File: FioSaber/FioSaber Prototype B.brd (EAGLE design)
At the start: 26.7 x 44.7 mm, 18 parts, among them P1 WIICHUCK, T1 2N2222

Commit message: labeled motor header
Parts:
- renumbered U$2 to MOTOR
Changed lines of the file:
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@@
 <element name="R4" library="adafruit" package="0207/7" value="33Ω" x="13.97" y="27.94" rot="R270"/>
 <element name="R3" library="adafruit" package="0207/7" value="1kΩ" x="11.43" y="27.94" rot="R90"/>
-<element name="U$2" library="headers(.1in)" package="1X2" value="1X2" x="11.43" y="35.56"/>
+<element name="MOTOR" library="headers(.1in)" package="1X2" value="1X2" x="11.43" y="35.56"/>
 <element name="D1" library="adafruit" package="DO41-10" value="1N4004" x="6.35" y="17.145" rot="R90"/>
 <element name="S1" library="adafruit" package="EG1218" value="" x="12.7" y="17.145" rot="R90"/>
@@
 <signal name="N$19">
 <contactref element="T1" pad="C"/>
-<contactref element="U$2" pad="1"/>
+<contactref element="MOTOR" pad="1"/>
 <contactref element="D2" pad="A"/>
 <contactref element="C1" pad="2"/>
@@
 </signal>
 <signal name="N$20">
-<contactref element="U$2" pad="2"/>
+<contactref element="MOTOR" pad="2"/>
 <contactref element="R4" pad="2"/>
 <contactref element="D2" pad="C"/>

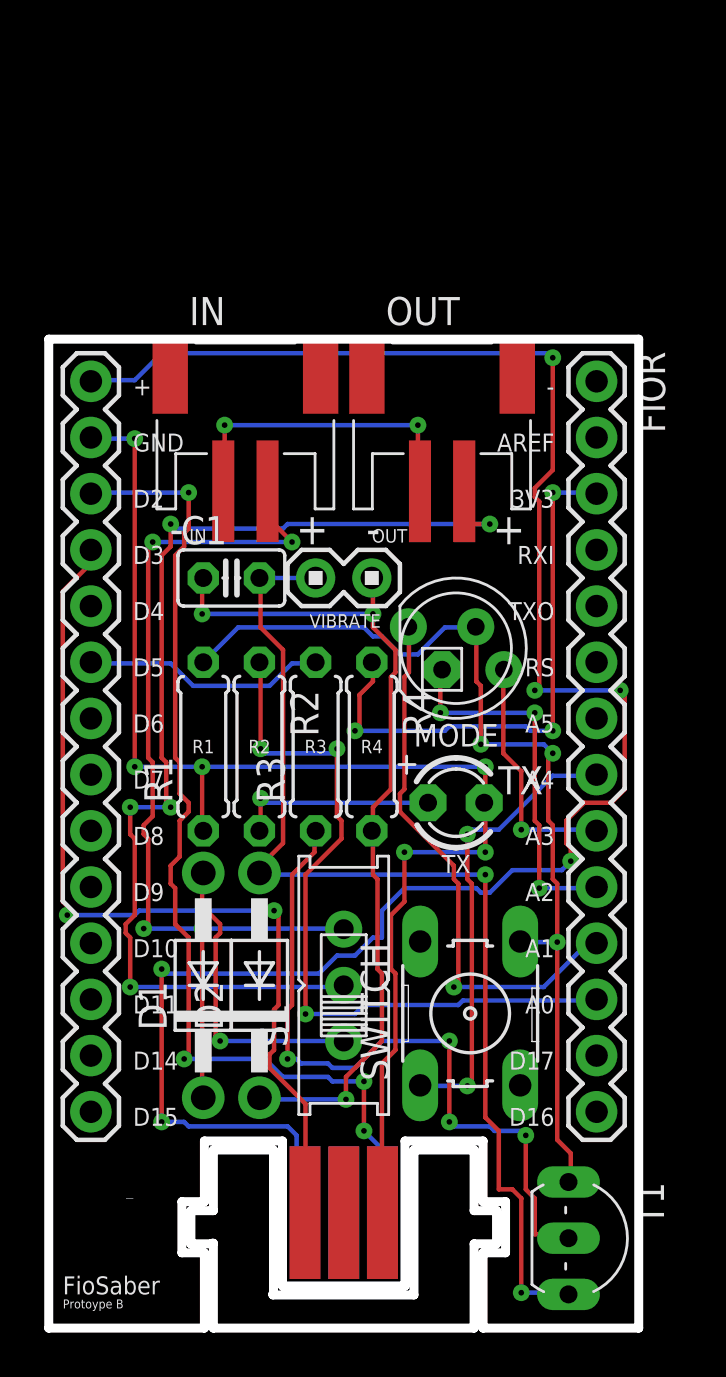
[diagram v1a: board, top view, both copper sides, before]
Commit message: reconfigured prototype b
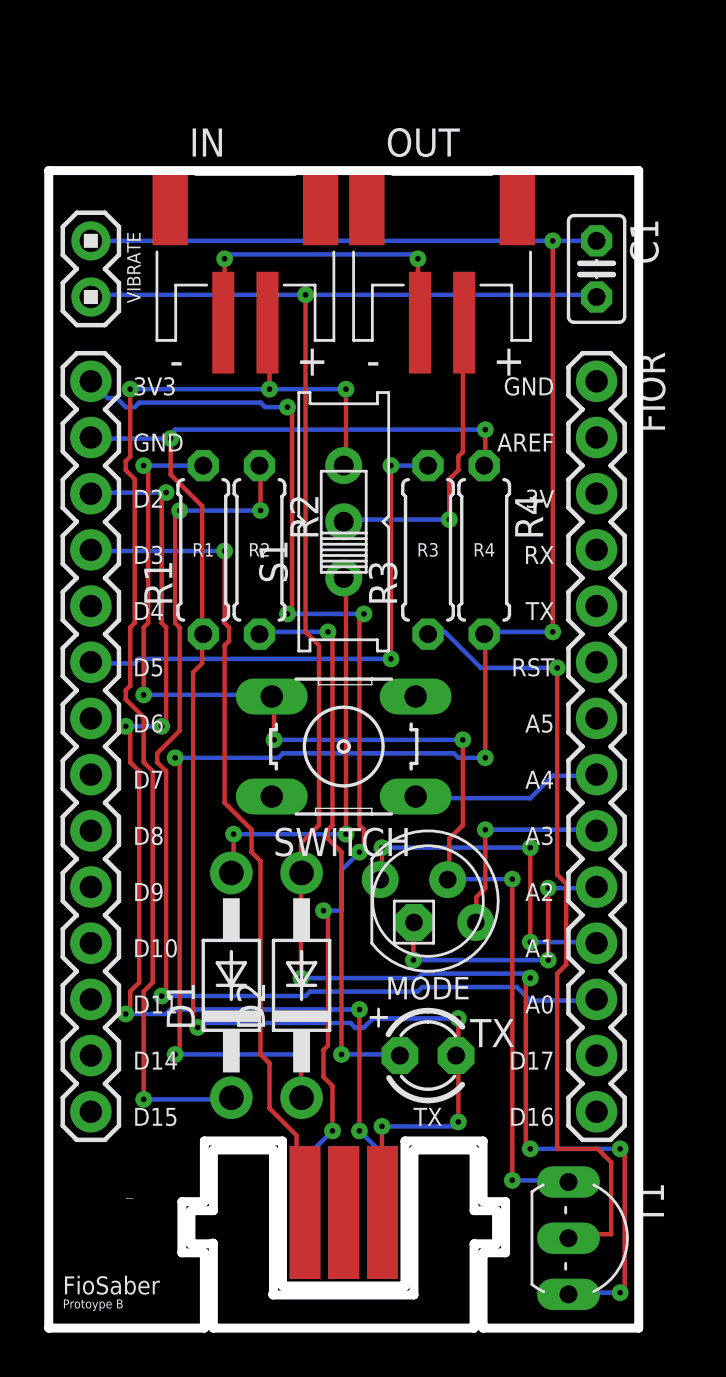
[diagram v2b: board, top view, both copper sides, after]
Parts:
- moved C1 21.6 mm to (24.1, 49.5), turned to 270 degrees
- moved S1 21.0 mm to (12.7, 38.1)
- moved MOTOR 16.3 mm to (1.27, 48.3), turned to 90 degrees
- moved SWITCH 13.4 mm to (12.7, 27.9), turned to 180 degrees
- moved MODE 11.5 mm to (16.5, 21.0)
- moved TX 11.5 mm to (16.5, 14.0)
- moved R3 10.2 mm to (16.5, 36.8)
- moved R4 10.2 mm to (19.1, 36.8)
- moved R1 8.89 mm to (6.35, 36.8)
- moved R2 8.89 mm to (8.89, 36.8)
- moved IN 7.62 mm to (8.26, 50.8)
- moved OUT 7.62 mm to (17.1, 50.8)
- moved D2 1.90 mm to (10.8, 17.1)
- moved D1 1.27 mm to (7.62, 17.1)
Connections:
- removed net N$12: FIOR.3, R4.1
- net N$9: now also R4.1
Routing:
- net N$20: track 38.7 -> 84.7 mm, vias 3 -> 6
- net N$1: track 89.2 -> 51.8 mm
- net N$19: track 49.1 -> 85.9 mm, vias 2 -> 6
- net N$10: track 50.4 -> 14.0 mm, vias 5 -> 1
- net N$12: track 25.3 -> 0.00 mm, vias 3 -> 0
- net N$25: track 9.15 -> 25.4 mm, vias 1 -> 2
- net N$17: track 33.7 -> 48.6 mm
- net N$16: track 11.0 -> 24.1 mm, vias 0 -> 2
- net N$14: track 20.6 -> 8.63 mm, vias 2 -> 0
- net N$9: track 60.0 -> 71.7 mm
- net N$13: track 44.4 -> 55.3 mm, vias 3 -> 6
- net N$2: track 43.7 -> 53.5 mm
- net N$6: track 24.9 -> 15.5 mm, vias 1 -> 3
- net N$5: track 13.7 -> 18.6 mm, vias 1 -> 2
- net N$18: track 32.4 -> 36.6 mm, vias 4 -> 1
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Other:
- board size 26.7 x 44.7 mm -> 26.7 x 52.3 mm
- board text added: "3V"
- board text added: "RST"
- board text added: "RX"
- board text removed: "+"
- board text removed: "-"
- board text removed: "IN"
- board text removed: "OUT"
- board text removed: "RS"
- board text removed: "RXI"
- board text removed: "TXO"

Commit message: prototype b tweaks
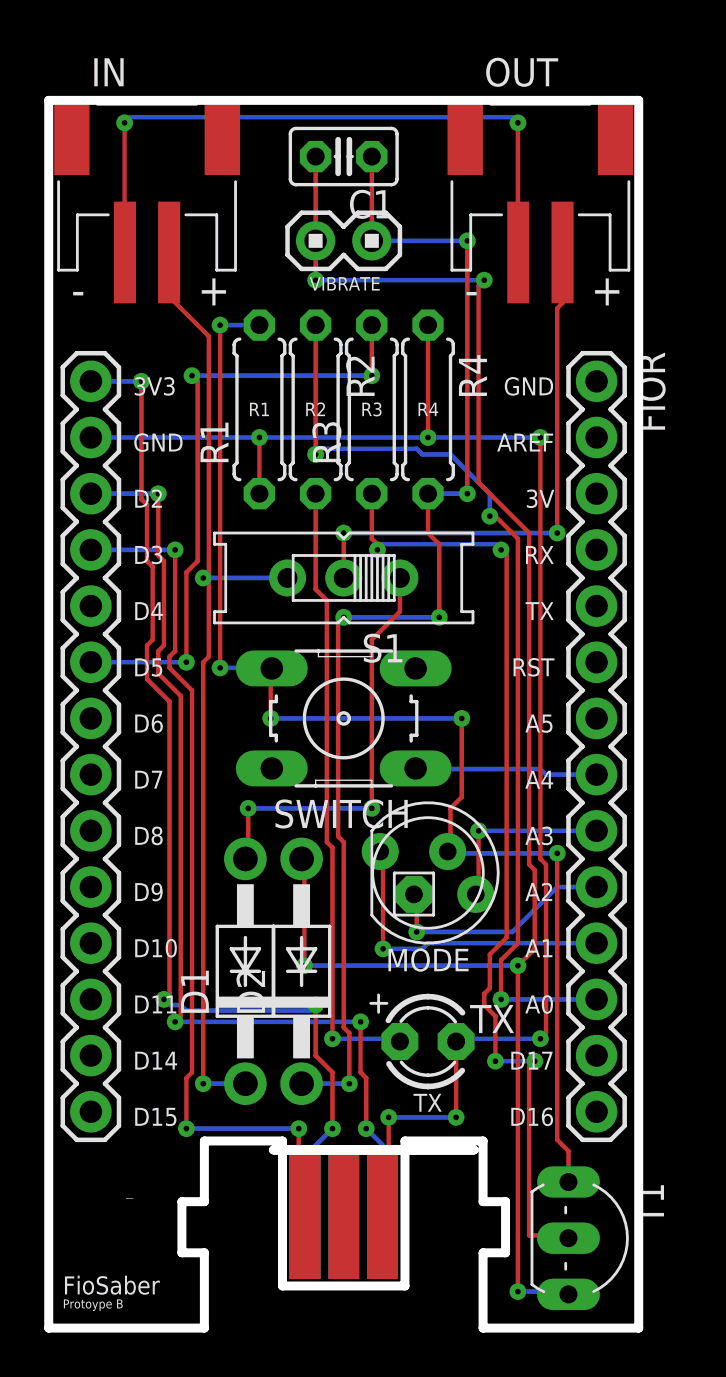
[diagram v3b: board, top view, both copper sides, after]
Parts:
- moved C1 12.5 mm to (12.7, 54.6), turned to 180 degrees
- moved MOTOR 10.5 mm to (11.4, 50.8), turned to 0 degrees
- moved R1 6.84 mm to (8.89, 43.2)
- moved R3 6.84 mm to (14.0, 43.2)
- moved R2 6.84 mm to (11.4, 43.2)
- moved R4 6.84 mm to (16.5, 43.2)
- moved IN 5.46 mm to (3.81, 54.0)
- moved OUT 5.46 mm to (21.6, 54.0)
- moved S1 2.54 mm to (12.7, 35.6), turned to 180 degrees
- moved MODE 1.27 mm to (16.5, 22.2)
- moved SWITCH 1.27 mm to (12.7, 29.2)
- moved D1 0.90 mm to (8.26, 17.8)
- moved D2 0.64 mm to (10.8, 17.8)
- moved TX 0.63 mm to (16.5, 14.6)
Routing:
- net N$20: track 84.7 -> 55.0 mm, vias 6 -> 5
- net N$11: track 14.8 -> 29.7 mm
- net N$10: track 14.0 -> 24.5 mm, vias 1 -> 2
- net N$2: track 53.5 -> 44.5 mm, vias 4 -> 2
- net N$19: track 85.9 -> 77.4 mm, vias 6 -> 5
- net N$18: track 36.6 -> 44.0 mm, vias 1 -> 4
- net N$17: track 48.6 -> 42.8 mm
- net N$3: track 49.6 -> 45.1 mm, vias 6 -> 4
- net N$16: track 24.1 -> 28.0 mm, vias 2 -> 3
- net N$1: track 51.8 -> 48.5 mm, vias 6 -> 4
- net N$25: track 25.4 -> 28.1 mm, vias 2 -> 1
- net N$7: track 13.2 -> 10.7 mm, vias 3 -> 1
- net N$4: track 37.7 -> 39.6 mm, vias 1 -> 3
- net N$9: track 71.7 -> 70.2 mm
- net N$13: track 55.3 -> 56.8 mm, vias 6 -> 5
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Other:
- board size 26.7 x 52.3 mm -> 26.7 x 55.5 mm
- board text added: "Bat In"
- board text removed: "Batt In"
